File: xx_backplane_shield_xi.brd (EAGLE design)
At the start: 41.6 x 43.2 mm, 14 parts

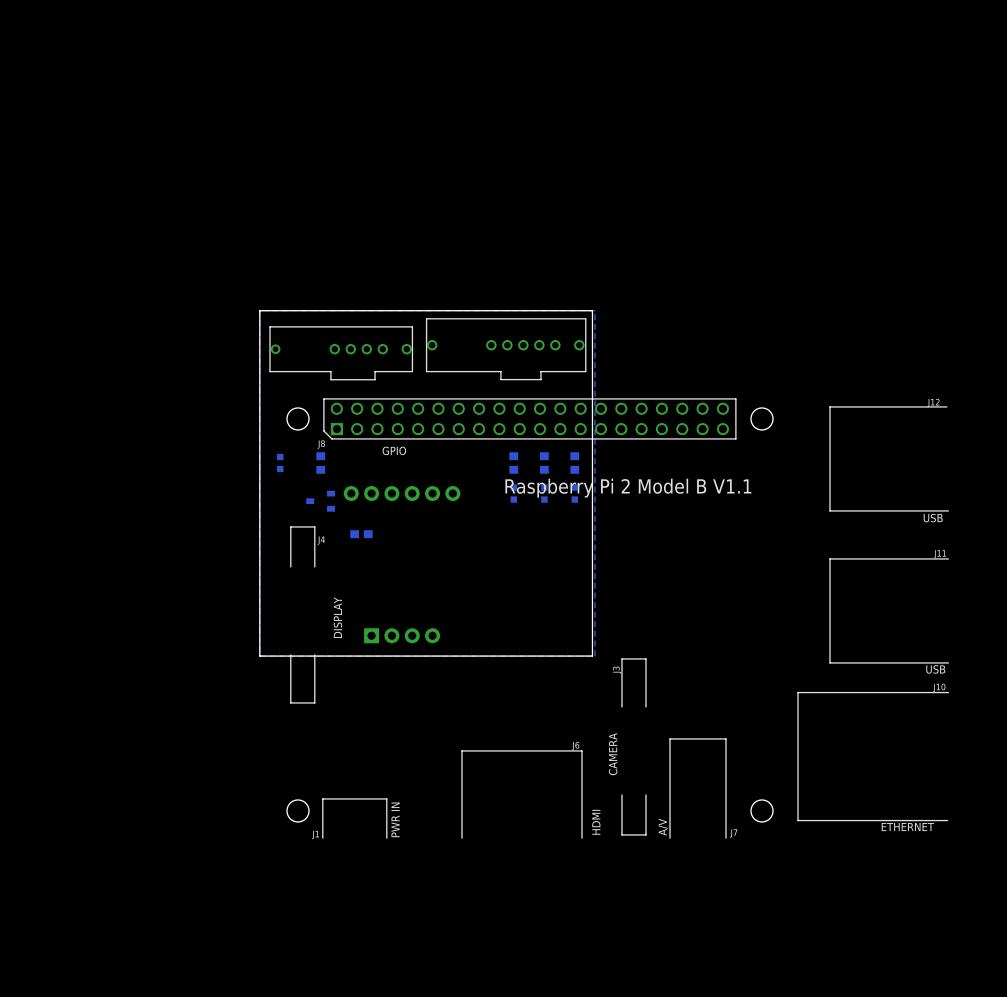
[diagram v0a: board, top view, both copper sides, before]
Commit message: finished board version 1
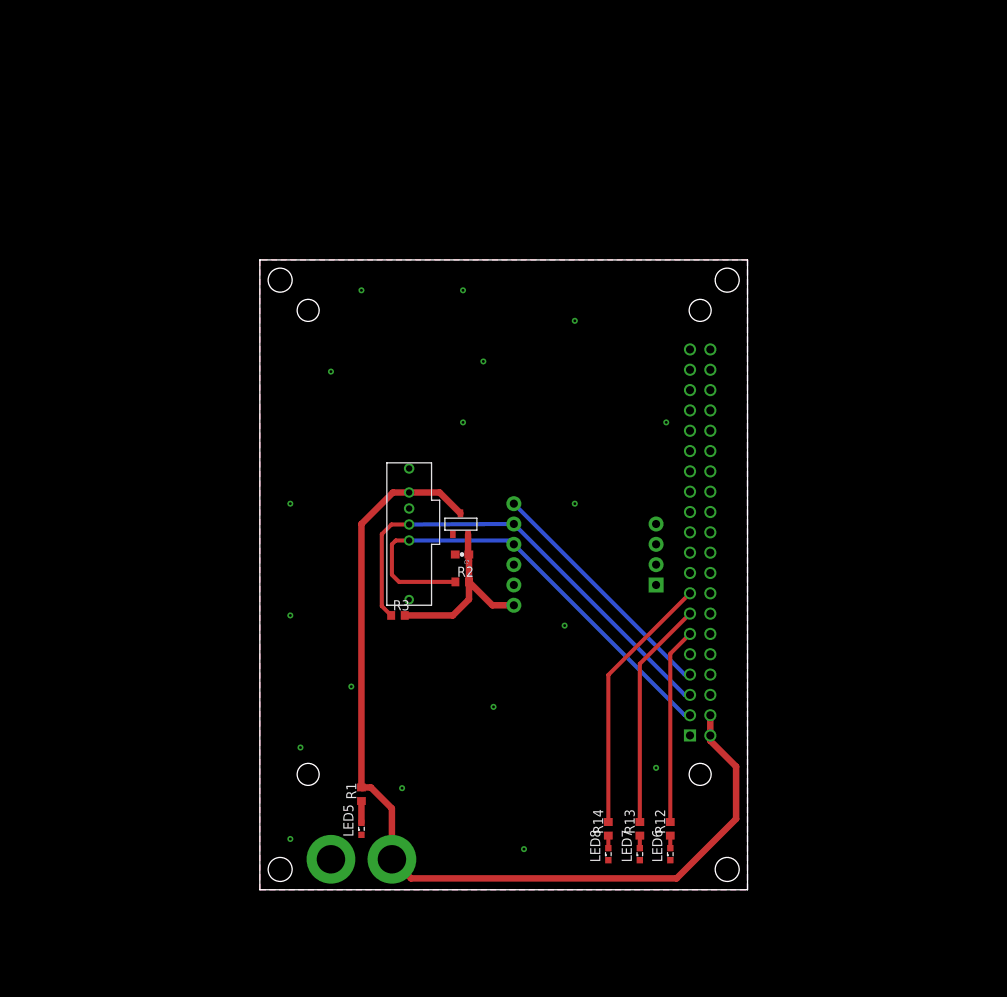
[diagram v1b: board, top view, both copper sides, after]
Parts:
- removed U$1: T2I, BackplaneParts:T2I
- added R2, R3: 330, resistor:R0603
- added U$4, U$6: THROUGHOLE, throughhole:THROUGHHOLE
- U$2: value T2I5P -> T2I; device BackplaneParts:T2I5P -> BackplaneParts:T2I
- moved R12 47.3 mm to (51.3, 7.62), flipped to the top
- moved R13 47.3 mm to (47.5, 7.62), flipped to the top
- moved R14 47.2 mm to (43.6, 7.62), flipped to the top
- moved LED5 46.8 mm to (12.7, 7.62), flipped to the top
- moved LED6 46.6 mm to (51.3, 4.45), flipped to the top
- moved LED7 46.6 mm to (47.5, 4.45), flipped to the top
- moved LED8 46.6 mm to (43.6, 4.45), flipped to the top
- moved R1 41.7 mm to (12.7, 11.9), flipped to the top, turned to 90 degrees
- moved U$2 34.9 mm to (21.5, 35.6), turned to 90 degrees
- moved U$3 24.1 mm to (40.6, 40.6), turned to 180 degrees
- moved U$5 16.1 mm to (24.1, 44.5), flipped to the top, turned to 0 degrees
- moved C7 12.8 mm to (25.3, 41.9), flipped to the top
- moved PCB1 4.75 mm to (2.54, 10.9), flipped to the bottom, turned to 90 degrees
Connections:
- removed net FIN: PCB1.P$33
- removed net LASER_ON: PCB1.P$29
- removed net MISO: PCB1.P$35
- removed net MOSI: PCB1.P$38
- removed net RX: PCB1.P$10
- removed net SCLK: PCB1.P$40
- removed net SERVO_PWM: PCB1.P$12
- removed net TX: PCB1.P$8
- net +5V: now also U$2.4, U$4.P$1; no longer U$2.P$5, U$2.P$6
- net 3.3V: now also R2.2, R3.2
- net GND: now also U$2.3, U$6.P$1; no longer U$2.P$2, U$2.P$3
- net LED1: now also PCB1.P$11; no longer PCB1.P$26
- net LED2: now also PCB1.P$13; no longer PCB1.P$24
- net LED3: now also PCB1.P$15; no longer PCB1.P$22
- net SCL: now also R3.1, U$2.2; no longer U$1.1
- net SDA: now also R2.1, U$2.1; no longer U$1.2
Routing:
- net +5V: track 0.00 -> 120.8 mm
- net SCL: track 0.00 -> 58.6 mm
- net SDA: track 0.00 -> 58.6 mm
- net LED3: track 0.00 -> 32.8 mm
- net RESET: track 0.00 -> 30.9 mm
- net LED2: track 0.00 -> 28.6 mm
- net LED1: track 0.00 -> 24.5 mm
- net 3.3V: track 0.00 -> 24.1 mm
- net N$2: track 0.00 -> 2.72 mm
- net N$15: track 0.00 -> 1.57 mm
- net N$14: track 0.00 -> 1.57 mm
- net N$13: track 0.00 -> 1.57 mm
- added copper zone on layer 1, net GND
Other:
- board size 41.6 x 43.2 mm -> 61 x 78.7 mm

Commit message: part placement almost done
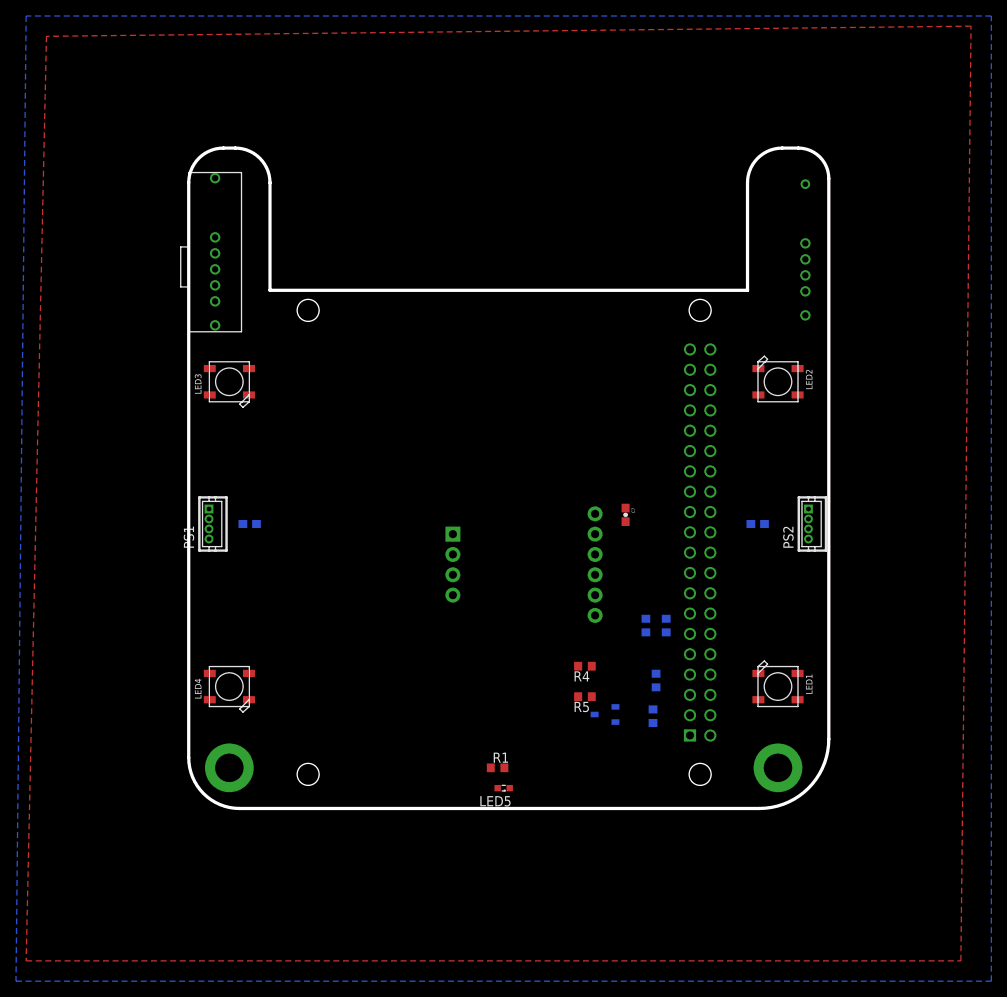
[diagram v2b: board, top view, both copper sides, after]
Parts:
- removed LED6, LED7, LED8: (no value), led:SML0603
- removed R12, R13, R14: 330, resistor:R0603
- added C1, C3: 0.1u, SparkFun-Passives:0603-CAP
- added LED1, LED2, LED3, LED4: WS2812B5050, microbuilder:WS2812B
- added POWER: T2I5P, T2I5P:T2I5P
- added PS1, PS2: DF13-4P-1.25DSA, con-hirose-df13:DF13-4P-1.25DSA
- added R4, R6: 0 Ohms, resistor:R0603
- added R5, R7: 0 ohms, resistor:R0603
- moved U$2 72.8 mm to (71.0, 88.9), flipped to the bottom, turned to 270 degrees
- moved U$4 49.6 mm to (64.8, 15.2)
- moved R3 33.3 mm to (49.5, 26.2), flipped to the bottom, turned to 90 degrees
- moved U$5 29.6 mm to (44.5, 22.9), flipped to the bottom, turned to 270 degrees
- moved R2 29.2 mm to (49.1, 21.7), flipped to the bottom, turned to 270 degrees
- moved C7 21.0 mm to (45.7, 46.9), turned to 270 degrees
- moved LED5 18.5 mm to (30.5, 12.7), turned to 180 degrees
- moved R1 17.3 mm to (29.7, 15.2), turned to 0 degrees
- moved U$6 17.1 mm to (-3.81, 15.2)
- moved U$3 7.73 mm to (33.0, 41.9), turned to 0 degrees
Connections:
- removed net BT_LED_ON: PCB1.P$36
- removed net LED_ON: PCB1.P$31
- removed net N$13: LED6.A, R12.1
- removed net N$14: LED7.A, R13.1
- removed net N$15: LED8.A, R14.1
- new net N$1: PS1.P$2, R4.2
- new net N$10: PS2.P$3, R7.2
- new net N$11: POWER.P$5
- new net N$12: POWER.P$6
- new net N$3: LED1.2-DOUT, LED2.4-DIN
- new net N$4: LED2.2-DOUT, LED3.4-DIN
- new net N$5: LED3.2-DOUT, LED4.4-DIN
- new net N$8: PS1.P$3, R5.2
- new net N$9: PS2.P$2, R6.2
- new net NEO_PIXEL_IN: LED1.4-DIN, PCB1.P$12
- net +5V: now also C1.1, C3.1, LED1.1-VDD, LED2.1-VDD, LED3.1-VDD, LED4.1-VDD; no longer U$2.4
- net 3.3V: now also PS1.P$1, PS2.P$1
- net GND: now also C1.2, C3.2, LED1.3-GND, LED2.3-GND, LED3.3-GND, LED4.3-GND, POWER.P$2, POWER.P$3, PS1.P$4, PS2.P$4; no longer LED6.C, LED7.C, LED8.C, U$2.3
- net LED1: no longer R12.2
- net LED2: no longer R13.2
- net LED3: no longer R14.2
- net SCL: now also R4.1, R6.1
- net SDA: now also R5.1, R7.1, U$2.3; no longer U$2.1
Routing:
- net +5V: track 120.8 -> 0.00 mm
- net SCL: track 58.6 -> 0.00 mm
- net SDA: track 58.6 -> 0.00 mm
- net LED3: track 32.8 -> 0.00 mm
- net RESET: track 30.9 -> 0.00 mm
- net LED2: track 28.6 -> 0.00 mm
- net LED1: track 24.5 -> 0.00 mm
- net 3.3V: track 24.1 -> 0.00 mm
- net N$2: track 2.72 -> 0.00 mm
- net N$15: track 1.57 -> 0.00 mm
- net N$14: track 1.57 -> 0.00 mm
- net N$13: track 1.57 -> 0.00 mm
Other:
- board size 61 x 78.7 mm -> 80 x 82.5 mm
